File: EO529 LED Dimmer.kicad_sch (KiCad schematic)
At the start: 35 parts, among them J1 VBat, Q1 BC639, Q2 BC639, Q3 BC639, Q4 BC639, U1 LM339, U2 NE555P

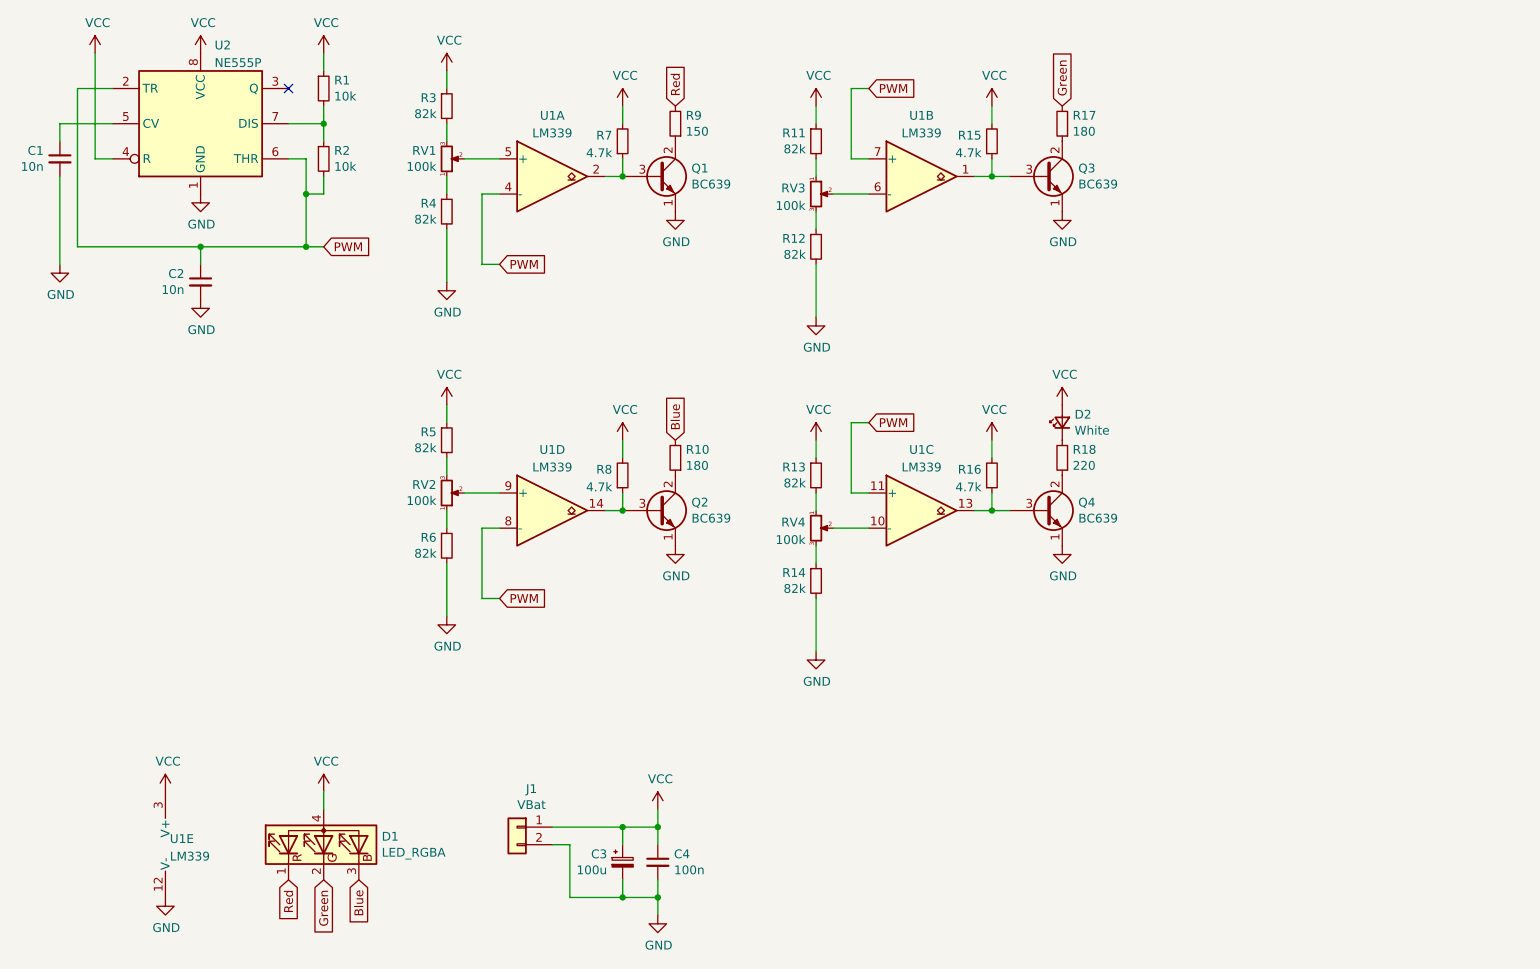
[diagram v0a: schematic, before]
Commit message: Revert "New layout, less parts"
This reverts commit 43836197f3911cfe2976812753205c060315a555.
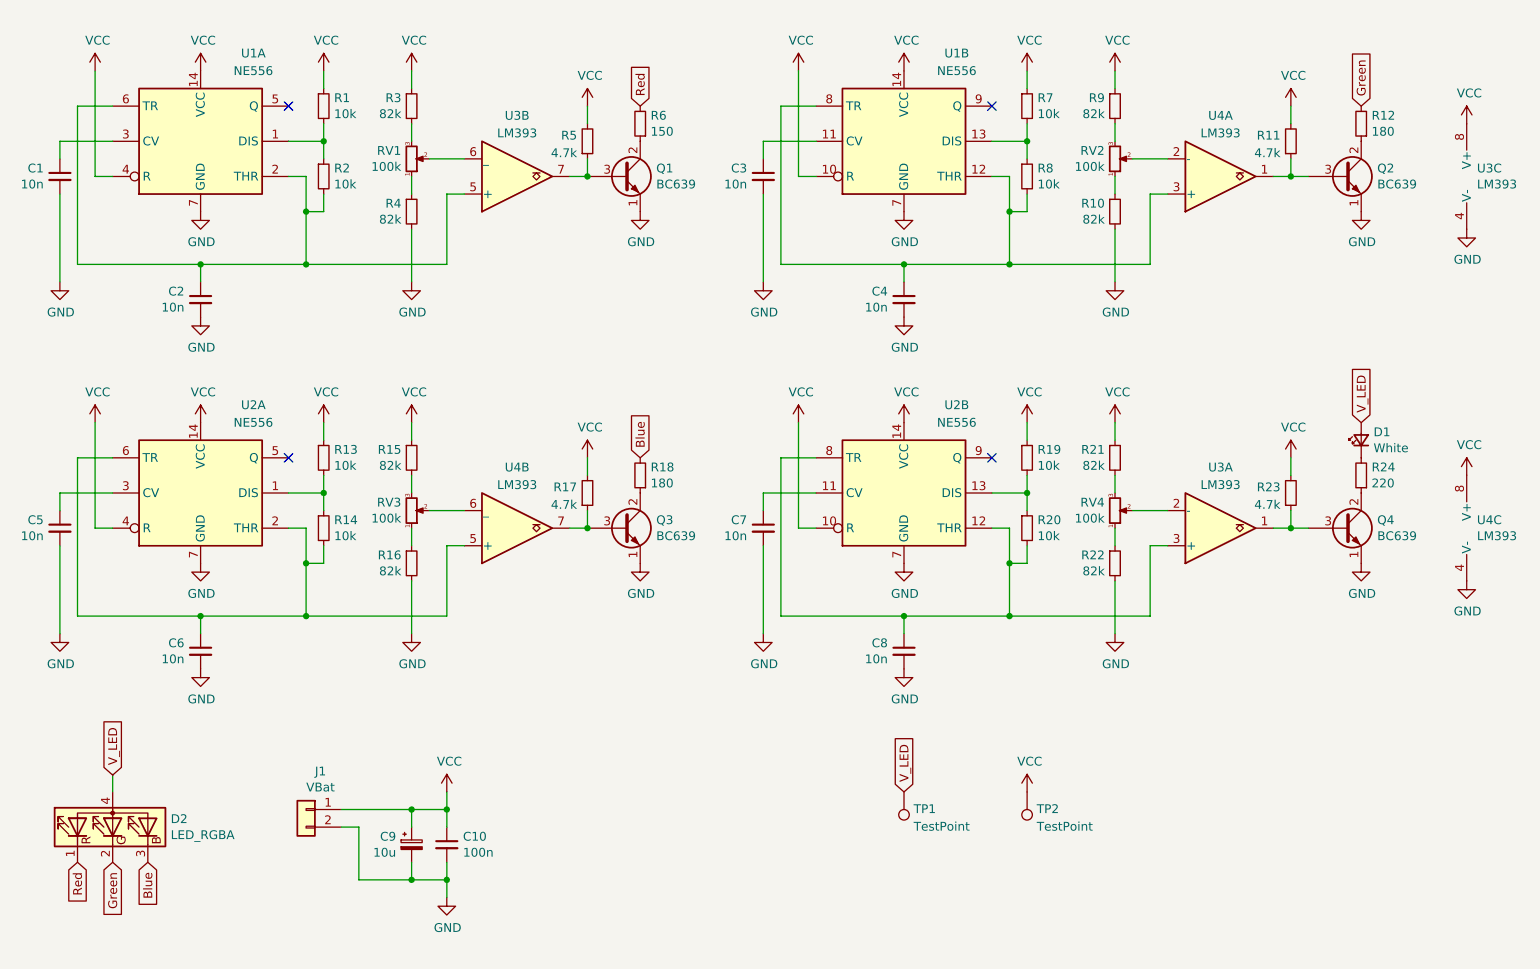
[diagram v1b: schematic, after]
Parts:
- removed U1: LM339, Package_DIP:DIP-14_W7.62mm_Socket, symbol Comparator:LM339
- removed U2: NE555P, Package_DIP:DIP-8_W7.62mm_Socket, symbol Timer:NE555P
- added C3, C4, C5, C6, C7, C8: 10n, Capacitor_THT:C_Disc_D5.0mm_W2.5mm_P5.00mm, symbol Device:C_Small
- added R13, R14, R19, R20, R7, R8: 10k, Resistor_THT:R_Axial_DIN0207_L6.3mm_D2.5mm_P7.62mm_Horizontal, symbol Device:R_Small
- added TP1, TP2: TestPoint, TestPoint:TestPoint_THTPad_D2.0mm_Drill1.0mm, symbol Connector:TestPoint
- added U1, U2: NE556, Package_DIP:DIP-14_W7.62mm_Socket, symbol Timer:NE556
- added U3, U4: LM393, Package_DIP:DIP-8_W7.62mm_Socket, symbol Comparator:LM393
- C9: renamed from C3; value 100u -> 10u; footprint Capacitor_THT:CP_Radial_D8.0mm_P3.50mm -> Capacitor_THT:CP_Radial_D5.0mm_P2.50mm
- Q1, Q4: footprint Package_TO_SOT_THT:TO-92_Inline_Wide -> Package_TO_SOT_THT:TO-92
- Q2: renamed from Q3; footprint Package_TO_SOT_THT:TO-92_Inline_Wide -> Package_TO_SOT_THT:TO-92
- Q3: renamed from Q2; footprint Package_TO_SOT_THT:TO-92_Inline_Wide -> Package_TO_SOT_THT:TO-92
- R12: renamed from R17; footprint Resistor_THT:R_Axial_DIN0207_L6.3mm_D2.5mm_P7.62mm_Horizontal -> Resistor_THT:R_Axial_DIN0414_L11.9mm_D4.5mm_P15.24mm_Horizontal
- R18: renamed from R10; footprint Resistor_THT:R_Axial_DIN0207_L6.3mm_D2.5mm_P7.62mm_Horizontal -> Resistor_THT:R_Axial_DIN0414_L11.9mm_D4.5mm_P15.24mm_Horizontal
- R24: renamed from R18; footprint Resistor_THT:R_Axial_DIN0207_L6.3mm_D2.5mm_P7.62mm_Horizontal -> Resistor_THT:R_Axial_DIN0414_L11.9mm_D4.5mm_P15.24mm_Horizontal
- R6: renamed from R9; footprint Resistor_THT:R_Axial_DIN0207_L6.3mm_D2.5mm_P7.62mm_Horizontal -> Resistor_THT:R_Axial_DIN0414_L11.9mm_D4.5mm_P15.24mm_Horizontal
- renumbered C4 to C10, D2 to D1, D1 to D2, R12 to R10, R15 to R11, R5 to R15, R6 to R16, R8 to R17, R13 to R21, R14 to R22, R16 to R23, R7 to R5, R11 to R9, RV3 to RV2, RV2 to RV3
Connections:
- net GND: now also C3.2, C4.2, C5.2, C6.2, C7.2, C8.2, U1.7 (GND), U1.7 (GND), U2.7 (GND), U2.7 (GND), U3.4 (V-), U4.4 (V-)
- net VCC: now also R13.1, R19.1, R7.1, TP2.1, U1.10 (R), U1.14 (VCC), U1.14 (VCC), U1.4 (R), U2.10 (R), U2.14 (VCC), U2.14 (VCC), U2.4 (R), U3.8 (V+), U4.8 (V+); no longer D1.2 (A), D2.4 (A)
- net at RV1.2: now also U3.6 (_)
- net at C1.1: now also U1.3 (CV)
- net at R1.2, R2.1: now also U1.1 (DIS)
- net at Q1.3 (B), R5.1: now also U3.7
- net at RV2.1: now also R10.1; no longer R9.2
- net at RV2.2: now also U4.2 (-)
- net at RV2.3: now also R9.2; no longer R10.1
- net at Q2.3 (B), R11.1: now also U4.1
- net at RV3.2: now also U4.6 (_)
- net at Q3.3 (B), R17.1: now also U4.7
- net at RV4.1: now also R22.1; no longer R21.2
- net at RV4.2: now also U3.2 (-)
- net at RV4.3: now also R21.2; no longer R22.1
- net at Q4.3 (B), R23.1: now also U3.1
- net PWM: no longer names the net of C2.1, R2.2
- net PWM: now also U1.2 (THR), U1.6 (TR), U3.5 (+)
- new net: C3.1, U1.11 (CV)
- new net: C4.1, R8.2, U1.12 (THR), U1.8 (TR), U4.3 (+)
- new net: R7.2, R8.1, U1.13 (DIS)
- new net: C6.1, R14.2, U2.2 (THR), U2.6 (TR), U4.5 (+)
- new net: R13.2, R14.1, U2.1 (DIS)
- new net: C5.1, U2.3 (CV)
- new net: C7.1, U2.11 (CV)
- new net: C8.1, R20.2, U2.12 (THR), U2.8 (TR), U3.3 (+)
- new net: R19.2, R20.1, U2.13 (DIS)
- new net V_LED: D1.2 (A), D2.4 (A), TP1.1
- no-connect marks 1 -> 4
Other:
- moved on the sheet: C1, C10, C2, C9, D1, D2, J1, Q1, Q2, Q3, Q4, R1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
